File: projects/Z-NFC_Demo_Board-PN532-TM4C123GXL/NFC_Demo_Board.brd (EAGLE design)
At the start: 100.5 x 51.7 mm, 5 parts, among them IC1 EK-TM4C123GXLP

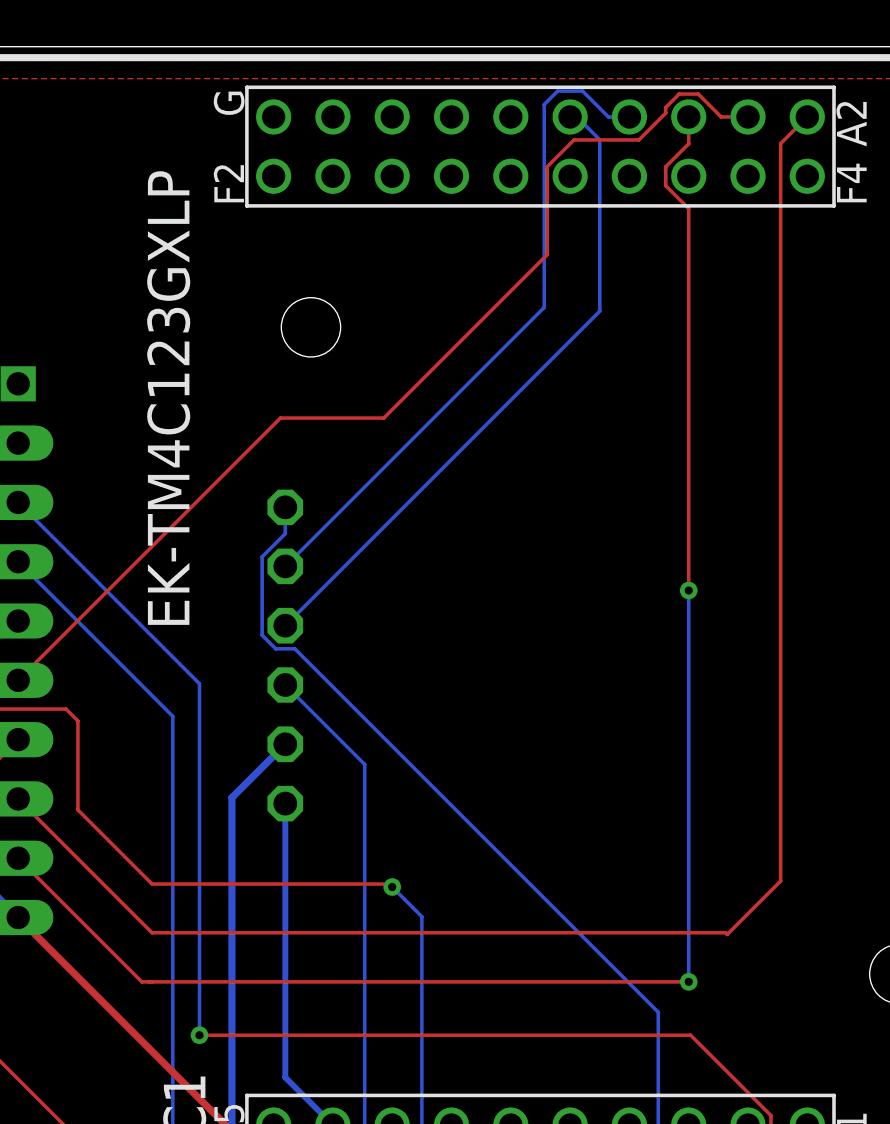
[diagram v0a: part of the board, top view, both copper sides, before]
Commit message: fixed some tiny inperfections
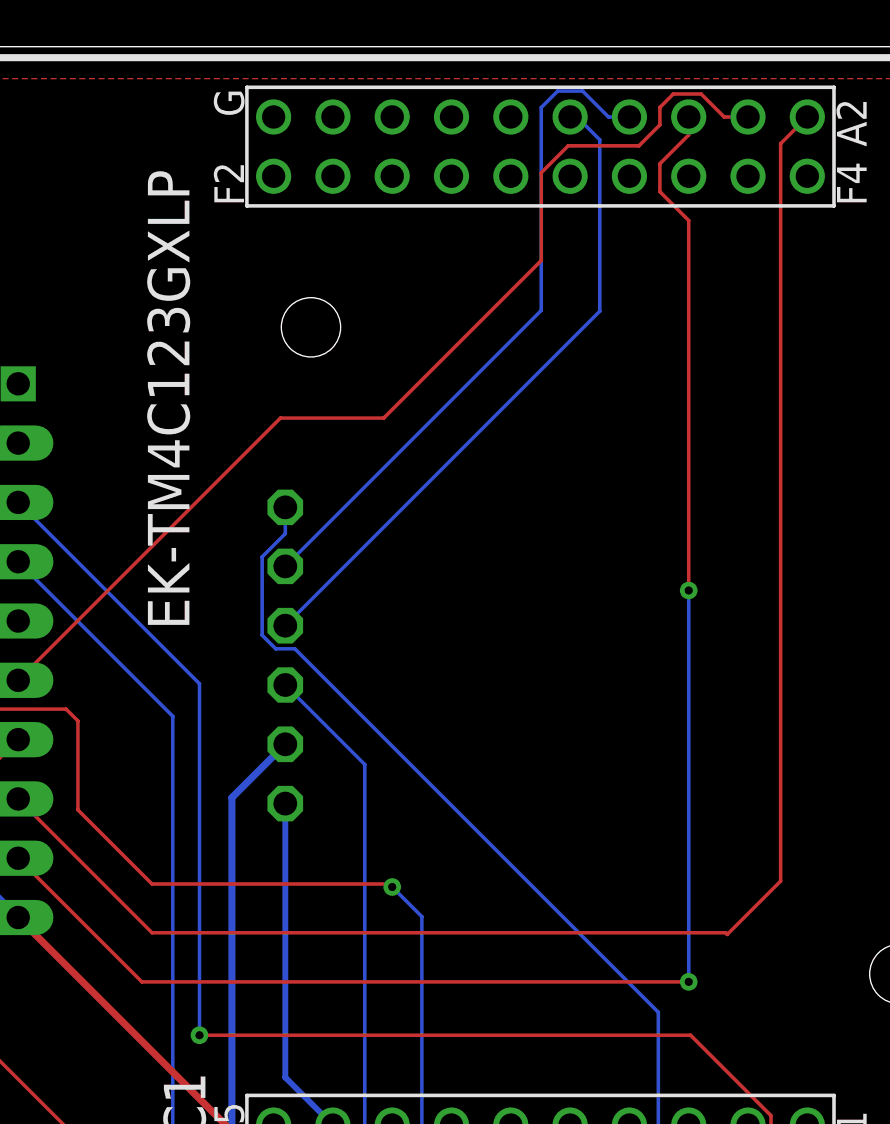
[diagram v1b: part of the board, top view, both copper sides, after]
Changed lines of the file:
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@@
 <contactref element="IC1" pad="12"/>
 <contactref element="DIS1" pad="6"/>
-<wire x1="131.0974" y1="73.26700625" x2="131.67299375" y2="73.8426" width="0.1524" layer="1"/>
-<wire x1="131.67299375" y1="73.8426" x2="132.48700625" y2="73.8426" width="0.1524" layer="1"/>
-<wire x1="131.0974" y1="73.02779375" x2="131.0974" y2="73.26700625" width="0.1524" layer="1"/>
-<wire x1="133.46960625" y1="72.86" x2="134.62" y2="72.86" width="0.1524" layer="1"/>
-<wire x1="129.94700625" y1="71.8774" x2="131.0974" y2="73.02779375" width="0.1524" layer="1"/>
-<wire x1="132.48700625" y1="73.8426" x2="133.46960625" y2="72.86" width="0.1524" layer="1"/>
-<wire x1="126.0174" y1="70.72700625" x2="127.16779375" y2="71.8774" width="0.1524" layer="1"/>
-<wire x1="127.16779375" y1="71.8774" x2="129.94700625" y2="71.8774" width="0.1524" layer="1"/>
+<wire x1="130.8434" y1="73.26700625" x2="131.41899375" y2="73.8426" width="0.1524" layer="1"/>
+<wire x1="131.41899375" y1="73.8426" x2="132.61400625" y2="73.8426" width="0.1524" layer="1"/>
+<wire x1="130.8434" y1="72.51979375" x2="130.8434" y2="73.26700625" width="0.1524" layer="1"/>
+<wire x1="133.59660625" y1="72.86" x2="134.62" y2="72.86" width="0.1524" layer="1"/>
+<wire x1="129.94700625" y1="71.6234" x2="130.8434" y2="72.51979375" width="0.1524" layer="1"/>
+<wire x1="132.61400625" y1="73.8426" x2="133.59660625" y2="72.86" width="0.1524" layer="1"/>
+<wire x1="125.7634" y1="70.47300625" x2="126.91379375" y2="71.6234" width="0.1524" layer="1"/>
+<wire x1="126.91379375" y1="71.6234" x2="129.94700625" y2="71.6234" width="0.1524" layer="1"/>
 <wire x1="103.36" y1="48.73" x2="114.5938" y2="59.9638" width="0.1524" layer="1"/>
 <wire x1="114.5938" y1="59.9638" x2="119.0188" y2="59.9638" width="0.1524" layer="1"/>
-<wire x1="119.0188" y1="59.9638" x2="126.0174" y2="66.9624" width="0.1524" layer="1"/>
-<wire x1="126.0174" y1="66.9624" x2="126.0174" y2="70.72700625" width="0.1524" layer="1"/>
+<wire x1="119.0188" y1="59.9638" x2="125.7634" y2="66.7084" width="0.1524" layer="1"/>
+<wire x1="125.7634" y1="66.7084" x2="125.7634" y2="70.47300625" width="0.1524" layer="1"/>
 </signal>
 <signal name="SSI0_MISO">
 <contactref element="IC1" pad="13"/>
 <contactref element="DIS1" pad="9"/>
-<wire x1="131.0974" y1="69.91299375" x2="131.0974" y2="70.72700625" width="0.1524" layer="1"/>
-<wire x1="132.08" y1="52.578" x2="132.08" y2="68.93039375" width="0.1524" layer="1"/>
-<wire x1="132.08" y1="71.70960625" x2="132.08" y2="72.86" width="0.1524" layer="1"/>
-<wire x1="132.08" y1="68.93039375" x2="131.0974" y2="69.91299375" width="0.1524" layer="1"/>
-<wire x1="131.0974" y1="70.72700625" x2="132.08" y2="71.70960625" width="0.1524" layer="1"/>
+<wire x1="130.8434" y1="69.65899375" x2="130.8434" y2="70.85400625" width="0.1524" layer="1"/>
+<wire x1="132.08" y1="52.578" x2="132.08" y2="68.42239375" width="0.1524" layer="1"/>
+<wire x1="132.08" y1="72.09060625" x2="132.08" y2="72.86" width="0.1524" layer="1"/>
+<wire x1="132.08" y1="68.42239375" x2="130.8434" y2="69.65899375" width="0.1524" layer="1"/>
+<wire x1="130.8434" y1="70.85400625" x2="132.08" y2="72.09060625" width="0.1524" layer="1"/>
 <via x="132.08" y="35.814" extent="1-16" drill="0.35"/>
-<wire x1="108.966" y1="35.814" x2="109.093" y2="35.814" width="0.1524" layer="1"/>
-<wire x1="109.093" y1="35.814" x2="132.08" y2="35.814" width="0.1524" layer="1"/>
+<wire x1="108.656" y1="35.814" x2="132.08" y2="35.814" width="0.1524" layer="1"/>
 <wire x1="132.08" y1="35.814" x2="132.08" y2="52.578" width="0.1524" layer="16"/>
 <via x="132.08" y="52.578" extent="1-16" drill="0.35"/>
 <wire x1="103.36" y1="41.11" x2="108.656" y2="35.814" width="0.1524" layer="1"/>
-<wire x1="108.656" y1="35.814" x2="108.966" y2="35.814" width="0.1524" layer="1"/>
 </signal>
 <signal name="SSI0_MOSI">
@@
 <contactref element="IC1" pad="14"/>
 <contactref element="U$1" pad="MISO"/>
-<wire x1="125.8904" y1="73.39400625" x2="126.46599375" y2="73.9696" width="0.1524" layer="16"/>
+<wire x1="125.7634" y1="73.26700625" x2="126.46599375" y2="73.9696" width="0.1524" layer="16"/>
 <wire x1="126.46599375" y1="73.9696" x2="127.53400625" y2="73.9696" width="0.1524" layer="16"/>
-<wire x1="114.8" y1="53.61" x2="125.8904" y2="64.7004" width="0.1524" layer="16"/>
+<wire x1="114.8" y1="53.61" x2="125.7634" y2="64.5734" width="0.1524" layer="16"/>
 <wire x1="128.64360625" y1="72.86" x2="129.54" y2="72.86" width="0.1524" layer="16"/>
 <wire x1="127.53400625" y1="73.9696" x2="128.64360625" y2="72.86" width="0.1524" layer="16"/>
-<wire x1="125.8904" y1="64.7004" x2="125.8904" y2="73.39400625" width="0.1524" layer="16"/>
+<wire x1="125.7634" y1="64.5734" x2="125.7634" y2="73.26700625" width="0.1524" layer="16"/>
 </signal>
 <signal name="SSI2_MOSI">
